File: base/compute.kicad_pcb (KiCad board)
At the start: 4 copper layers, 88.4 x 63.6 mm, 125 parts, among them IC1 TMC2209-LA-T, IC2 TMC2209-LA-T, IC3 TMC2209-LA-T, IC4 DMP6023LSS-13, J1 USB_C_Receptacle_USB2.0_16P, J13 fan, J2 FPC-24P-0.5mm, J3 2-84952-0, J4 DC_Jack_5.5x2.5, J9 spindle, Q1 Q_NMOS_GDS_spindle, Q2 Q_NMOS_GSD_fan, SW1 SW_Push_Open, SW2 SW_Push_Open, U1 MCP1700T-1202ETT, U2 ESP32-S3-WROOM-2, U3 LM1117MPX-5.0/NOPB, U4 MCP1700-1502, U5 ICE40UP5K-SG48ITR-FPGA_Lattice, U6 MCP1700T-2802E, U7 USBLC6-2SC6, U8 AP63203WU-7

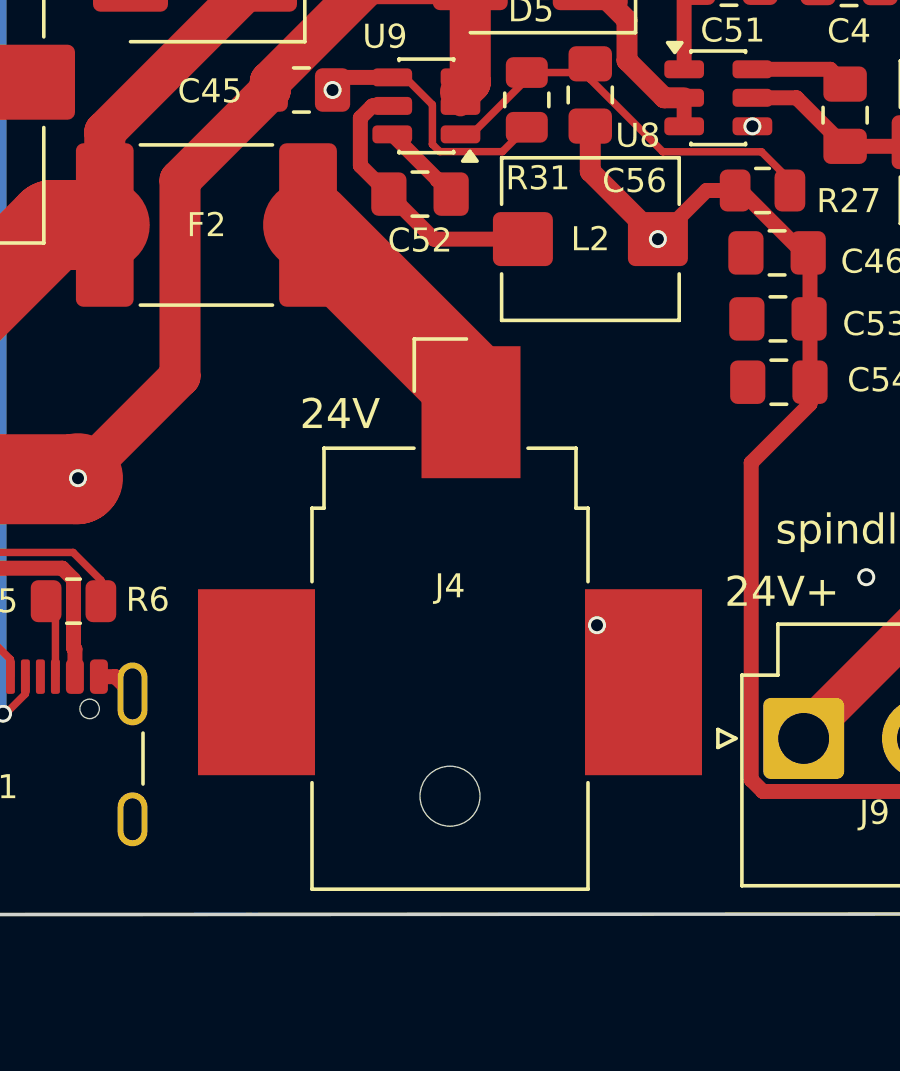
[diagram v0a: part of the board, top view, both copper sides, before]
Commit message: small fix compute pcb
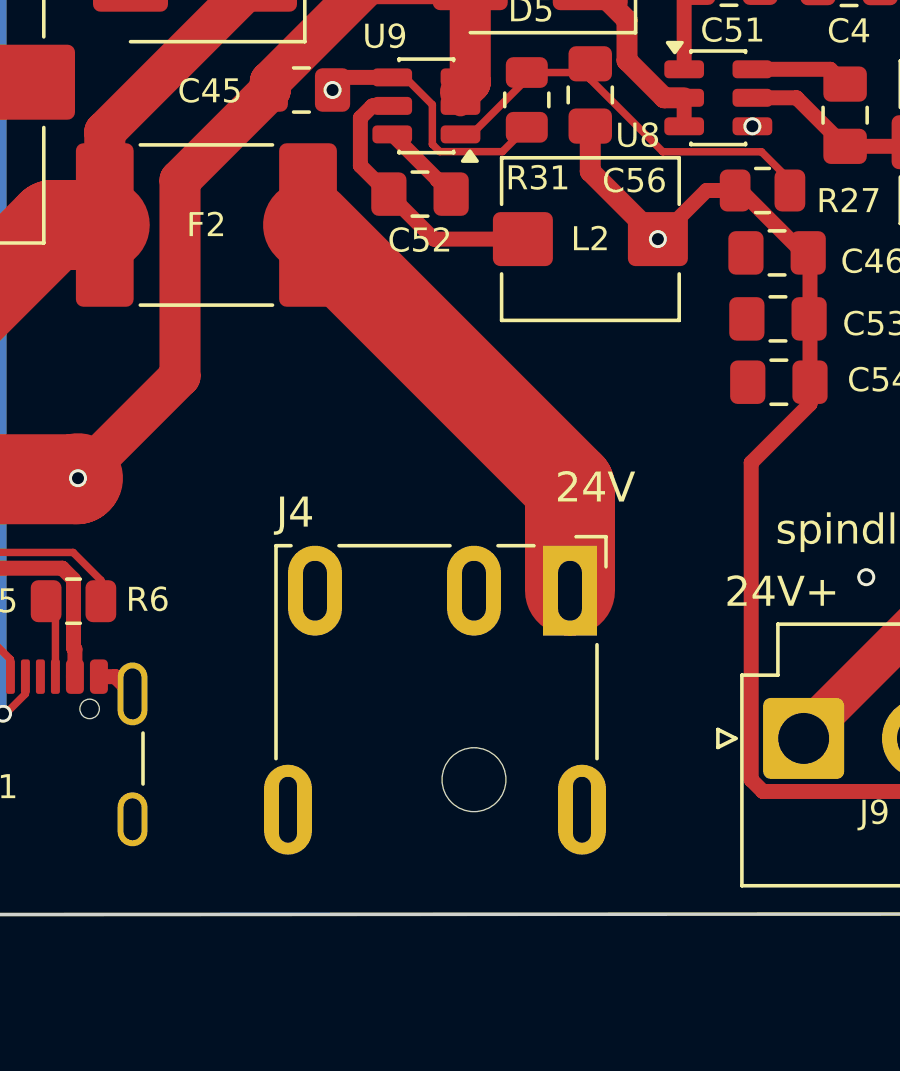
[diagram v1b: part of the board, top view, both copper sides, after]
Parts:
- J2: value FPC-24P-0.5mm -> FH12A-24S-0.5SH
- J4: footprint footprints:BarrelJack_CUI_PJ-036AH-SMT_Horizontal -> Connector_BarrelJack:BarrelJack_CUI_PJ-079BH_Horizontal
- R8, R9: value 5.1K -> 1.5K
- moved J4 4.00 mm to (200.5, 183.8)
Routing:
- net Net-(F2-Pad2): track 8.49 -> 15.8 mm
- net GND: vias 38 -> 37
